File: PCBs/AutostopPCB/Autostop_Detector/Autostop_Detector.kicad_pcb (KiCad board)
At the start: 2 copper layers, 52 x 100 mm, 15 parts, among them J5 DSUB9 to backplane, P1 282837-2, U1 ESP32-S3-DevKitC, U2 SN65HVD230

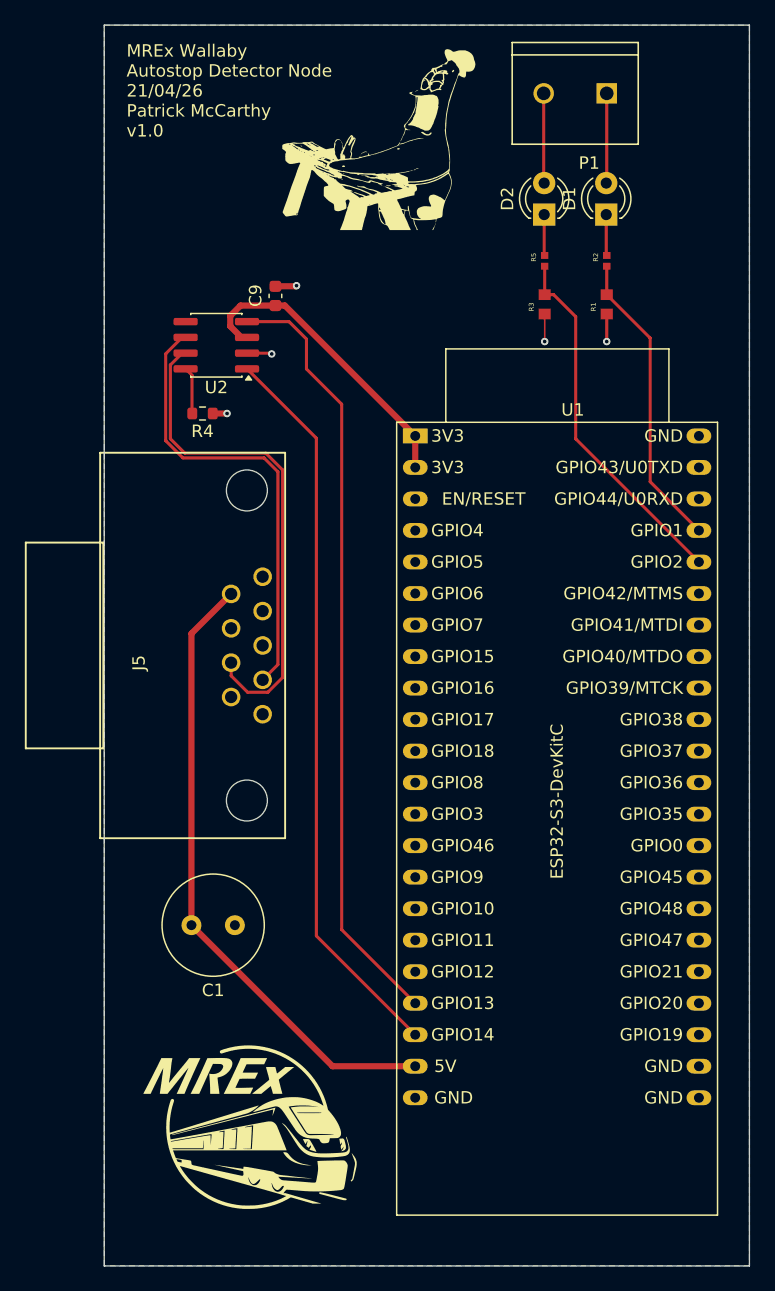
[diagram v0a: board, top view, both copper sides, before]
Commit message: Revert "added driver controls v2"
This reverts commit c73e8f860f70517a898f0b3e351800c05ab551df.
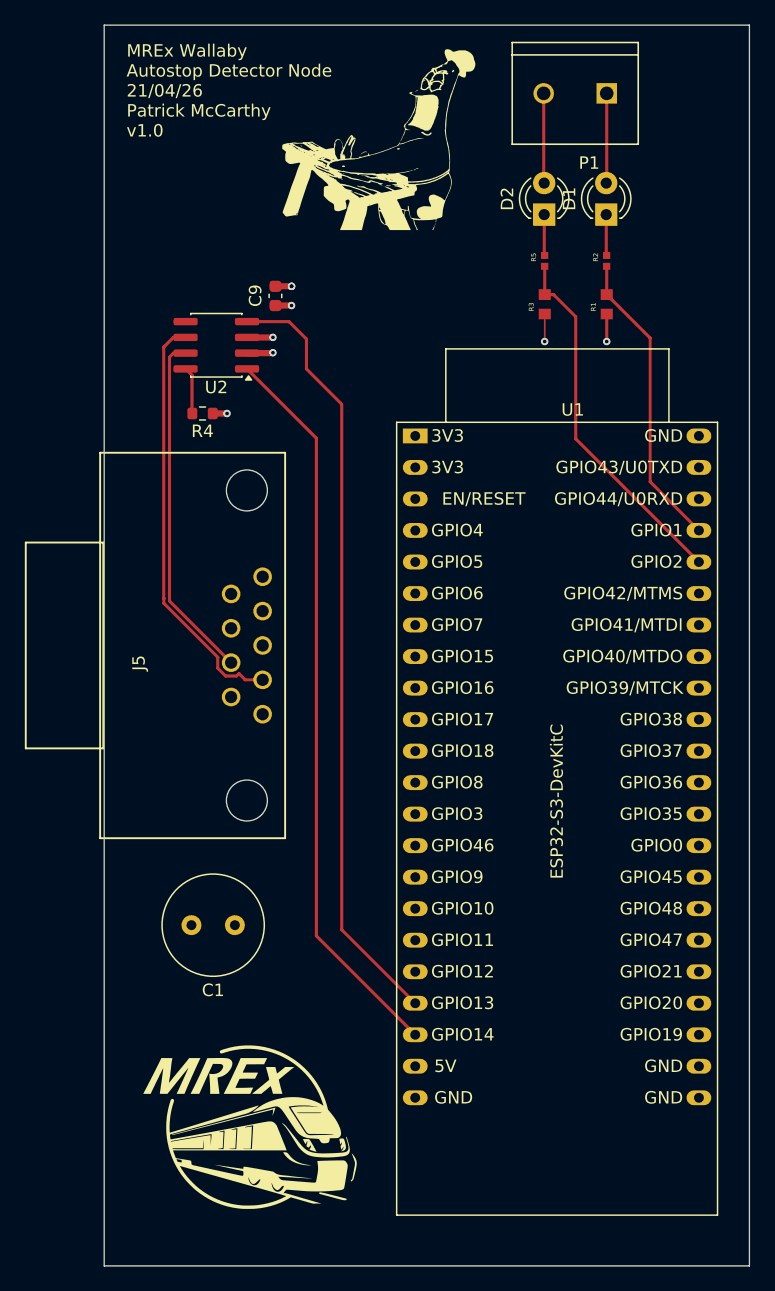
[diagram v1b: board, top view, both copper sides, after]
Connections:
- R1 pad 2: Net-(U1-GPIO1/ADC1_CH0) -> unconnected-(R1-Pad2)
- R2 pad 1: Net-(U1-GPIO1/ADC1_CH0) -> unconnected-(R1-Pad2)
- R3 pad 2: Net-(U1-GPIO2/ADC1_CH1) -> unconnected-(R3-Pad2)
- R5 pad 1: Net-(U1-GPIO2/ADC1_CH1) -> unconnected-(R3-Pad2)
- U1 pad 40: Net-(U1-GPIO2/ADC1_CH1) -> unconnected-(R3-Pad2)
- U1 pad 41: Net-(U1-GPIO1/ADC1_CH0) -> unconnected-(R1-Pad2)
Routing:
- net GND: track 9.35 -> 151.3 mm, vias 5 -> 6
- net unconnected-(R3-Pad2): track 0.00 -> 29.4 mm
- net Net-(U1-GPIO2/ADC1_CH1): track 29.4 -> 0.00 mm
- net unconnected-(R1-Pad2): track 0.00 -> 24.4 mm
- net Net-(U1-GPIO1/ADC1_CH0): track 24.4 -> 0.00 mm
- net /CANH: track 40.6 -> 28.1 mm
- net +3V3: track 24.7 -> 29.4 mm, vias 0 -> 2
- net /CANL: track 36.5 -> 33.9 mm
- added copper zone on In1.Cu, net GND
- removed copper zone on B.Cu, net GND
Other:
- copper layers 2 -> 4
